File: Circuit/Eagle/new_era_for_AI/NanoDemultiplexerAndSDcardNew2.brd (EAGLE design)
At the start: 94 x 70 mm, 31 parts

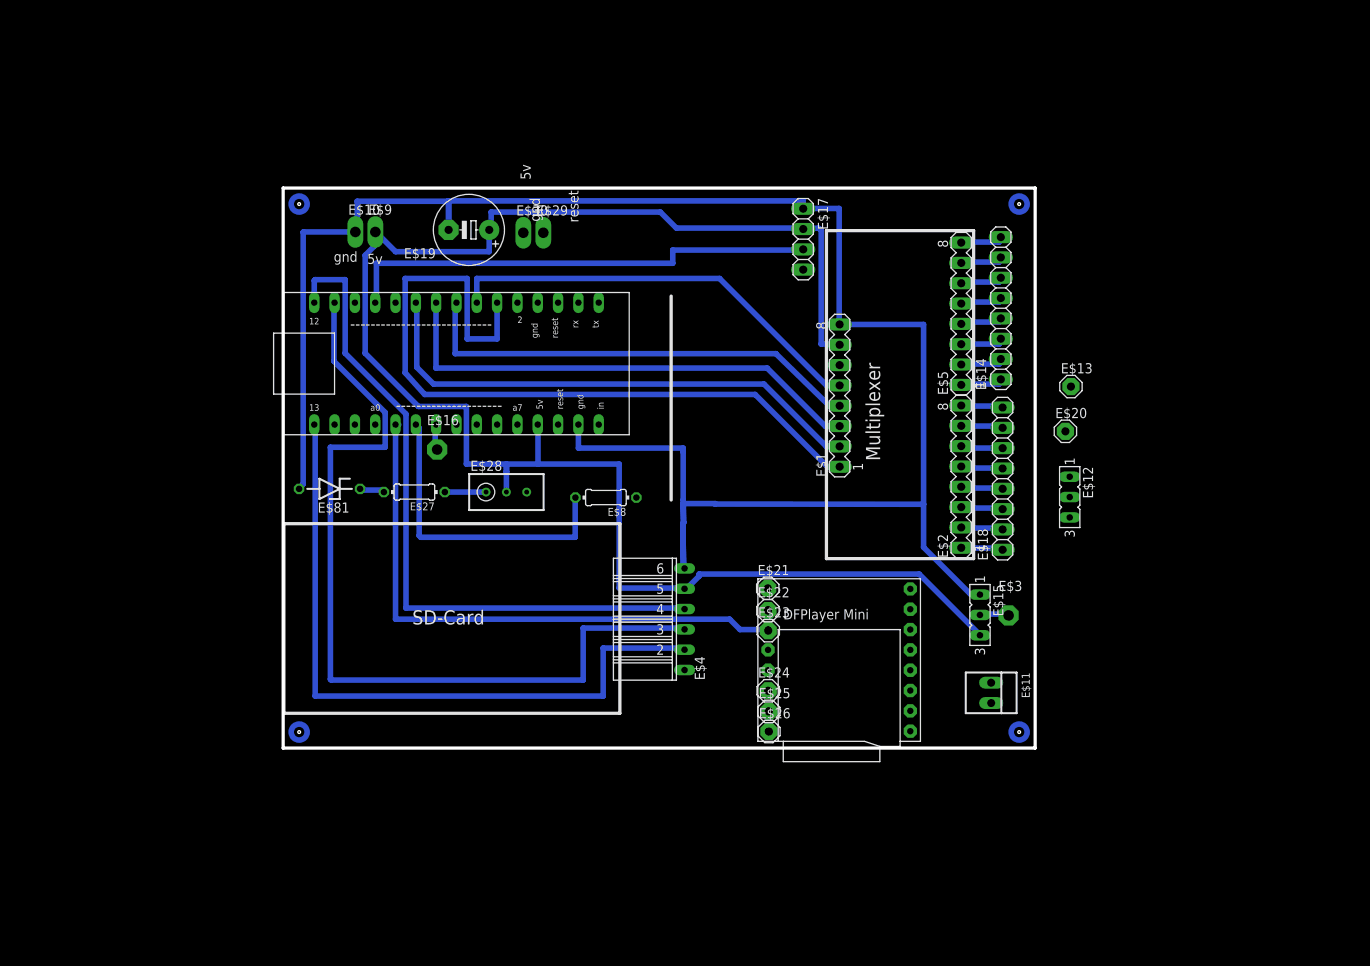
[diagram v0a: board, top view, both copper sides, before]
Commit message: .
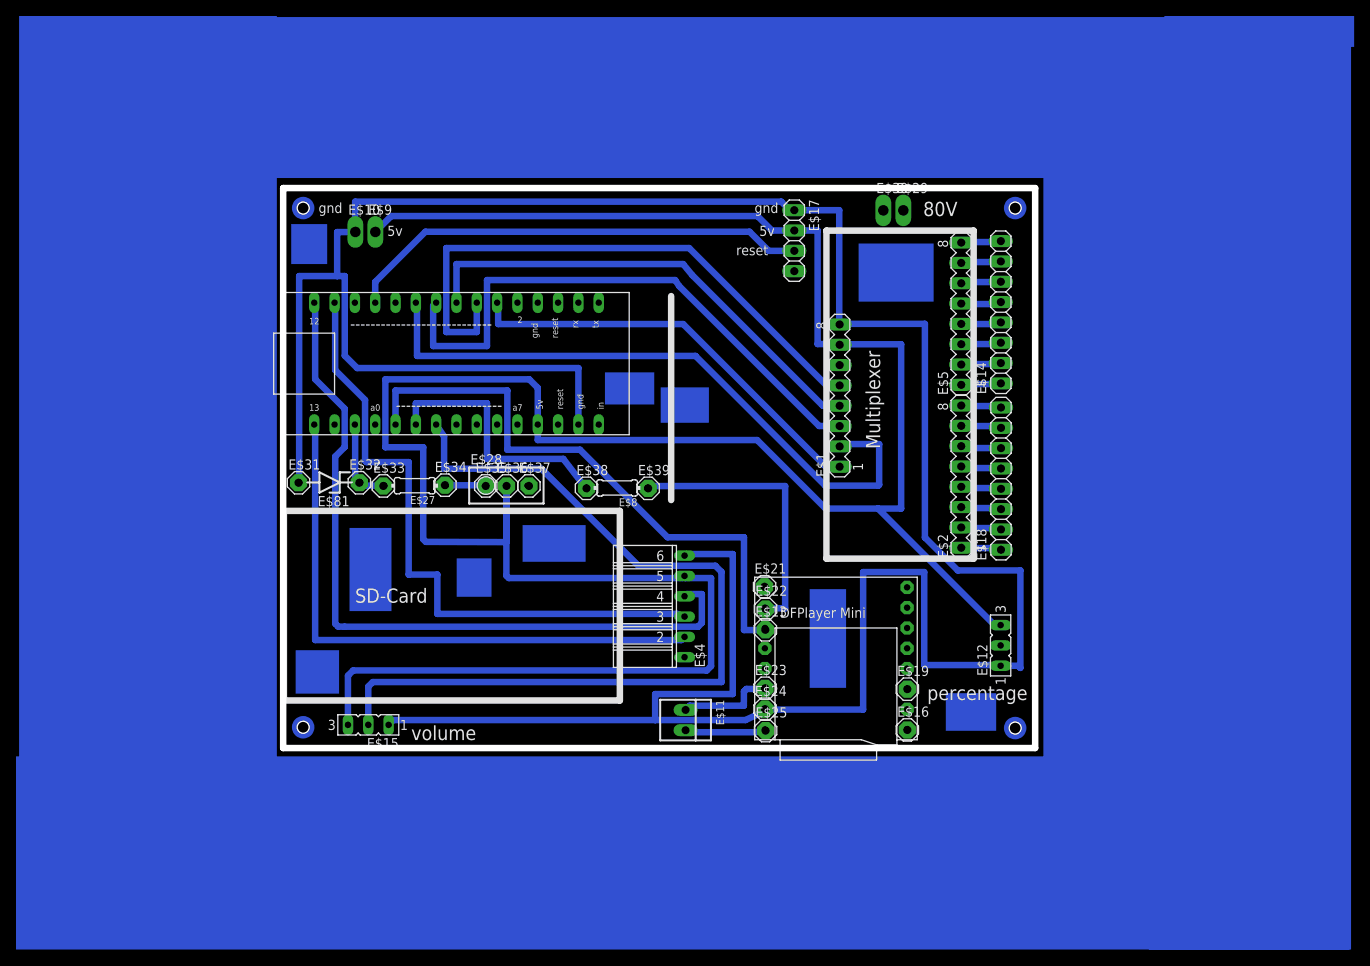
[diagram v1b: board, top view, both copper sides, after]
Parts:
- removed E$20, E$26: (no value), solpad:MCS10B
- removed E$3: (no value), discrete:PAD-01
- added E$31, E$32, E$33, E$34, E$35, E$36, E$37, E$38, E$39: (no value), solpad:MCS10B
- E$16: device discrete:PAD-01 -> solpad:MCS10B
- E$19: value 1000uF -> (none); device ref-packages-longpad:E5-8,5 -> solpad:MCS10B
- E$27: value 2.2K -> 50
- E$81: value zener 3.9v -> zener 4.3v
- moved E$15 79.8 mm to (14.1, 4.90), turned to 180 degrees
- moved E$19 79.4 mm to (84.0, 9.36), turned to 0 degrees
- moved E$16 68.4 mm to (84.0, 4.26)
- moved E$13 48.8 mm to (66.3, 16.8)
- moved E$29 45.1 mm to (83.5, 69.2)
- moved E$30 45.1 mm to (81.0, 69.2)
- moved E$11 38.4 mm to (56.3, 5.50)
- moved E$12 16.0 mm to (95.7, 17.4), turned to 90 degrees
- moved E$23 7.21 mm to (66.2, 9.48)
- moved E$25 2.43 mm to (66.3, 4.18)
- moved E$24 2.33 mm to (66.2, 6.86)
- moved E$8 1.84 mm to (47.7, 34.5)
- moved E$4 1.60 mm to (56.2, 19.7)
- moved E$17 1.13 mm to (69.9, 65.4)
- moved E$28 0.82 mm to (33.9, 34.8)
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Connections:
- net S$30 renamed RESET
- new net S$4: E$12.2, E$7.P$46
- net 5V: now also E$12.5; no longer E$19.+
- net GND: now also E$12.1; no longer E$19.-
- net S$2: now also E$7.P$35
- net VOLUME-CONTROL: no longer E$16.1, E$3.1
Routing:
- net 5V: track 210.6 -> 341.4 mm
- net GND: track 243.0 -> 373.6 mm
- net VOLUME-CONTROL: track 6.96 -> 108.8 mm
- net SIGN: track 94.6 -> 52.8 mm
- net RX: track 0.00 -> 35.1 mm
- net MOSI: track 107.5 -> 80.4 mm
- net S0: track 53.9 -> 74.3 mm
- net S3: track 65.1 -> 81.5 mm
- net SCK: track 86.4 -> 73.3 mm
- net SPK1: track 0.00 -> 12.0 mm
- net S2: track 61.7 -> 72.3 mm
- net SPK2: track 0.00 -> 10.1 mm
- net MISO: track 85.7 -> 94.2 mm
- net S$2: track 3.30 -> 10.6 mm
- net S$10: track 38.6 -> 32.7 mm
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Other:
- board text added: "80V"
- board text added: "percentage"
- board text added: "volume"
